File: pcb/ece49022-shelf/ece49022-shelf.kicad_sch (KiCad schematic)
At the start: 10 parts, among them J2 Conn_01x16_Pin, J3 Conn_01x04_Pin, J6 Conn_01x02_Pin, J7 Conn_01x02_Pin

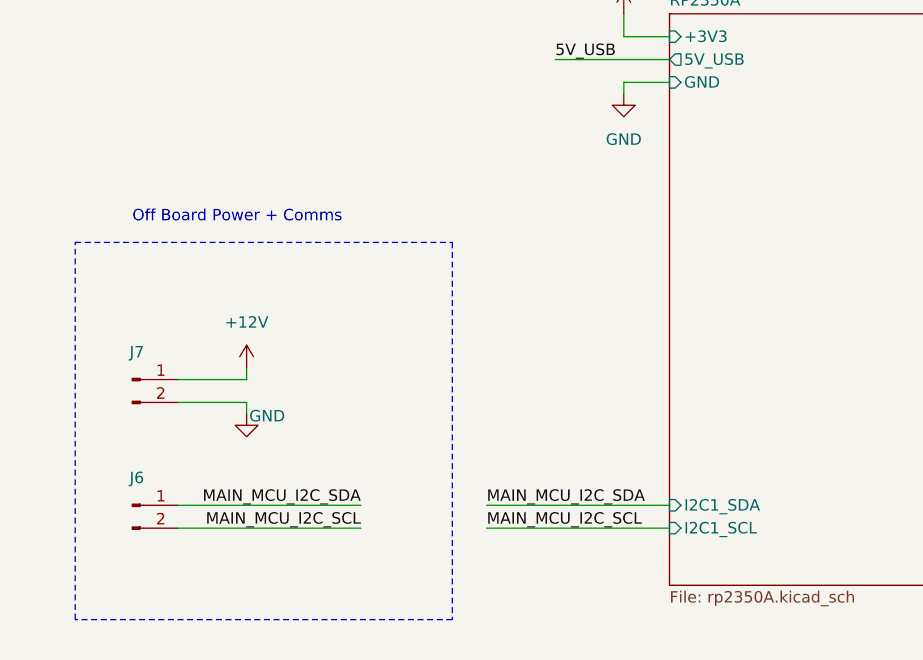
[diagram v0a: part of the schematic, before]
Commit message: stuff
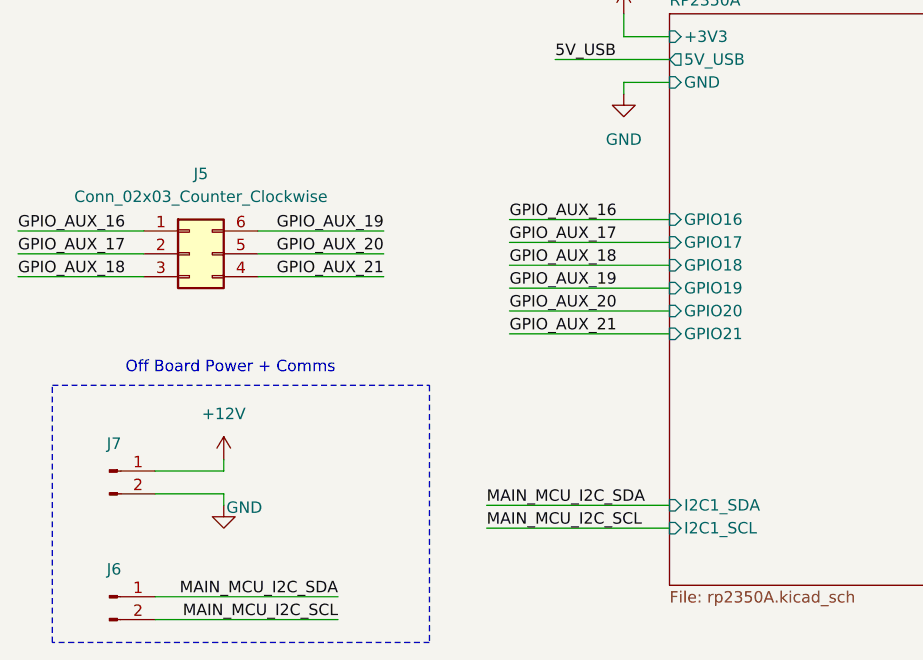
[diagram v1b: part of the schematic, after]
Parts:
- added J5: Conn_02x03_Counter_Clockwise, Connector_PinHeader_2.54mm:PinHeader_2x03_P2.54mm_Vertical, symbol Connector_Generic:Conn_02x03_Counter_Clockwise
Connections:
- new net GPIO_AUX_16: J5.1 (Pin_1)
- new net GPIO_AUX_17: J5.2 (Pin_2)
- new net GPIO_AUX_18: J5.3 (Pin_3)
- new net GPIO_AUX_19: J5.6 (Pin_6)
- new net GPIO_AUX_20: J5.5 (Pin_5)
- new net GPIO_AUX_21: J5.4 (Pin_4)
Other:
- sheet RP2350A ports: added GPIO16, GPIO17, GPIO18, GPIO19, GPIO20, GPIO21; removed none
- moved on the sheet: J6, J7
